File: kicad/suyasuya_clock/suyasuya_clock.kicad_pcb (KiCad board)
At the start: 2 copper layers, 66 x 78.7 mm, 33 parts, among them J1 Jack-DC, J2 Conn_Writer, J3 Conn_GPS, J4 USB_OUTPUT, Q1 2sk4017, SW1 RESET, U1 ATmega328-P, U2 BA50DD0T, U3 7803, Y1 Ceralock

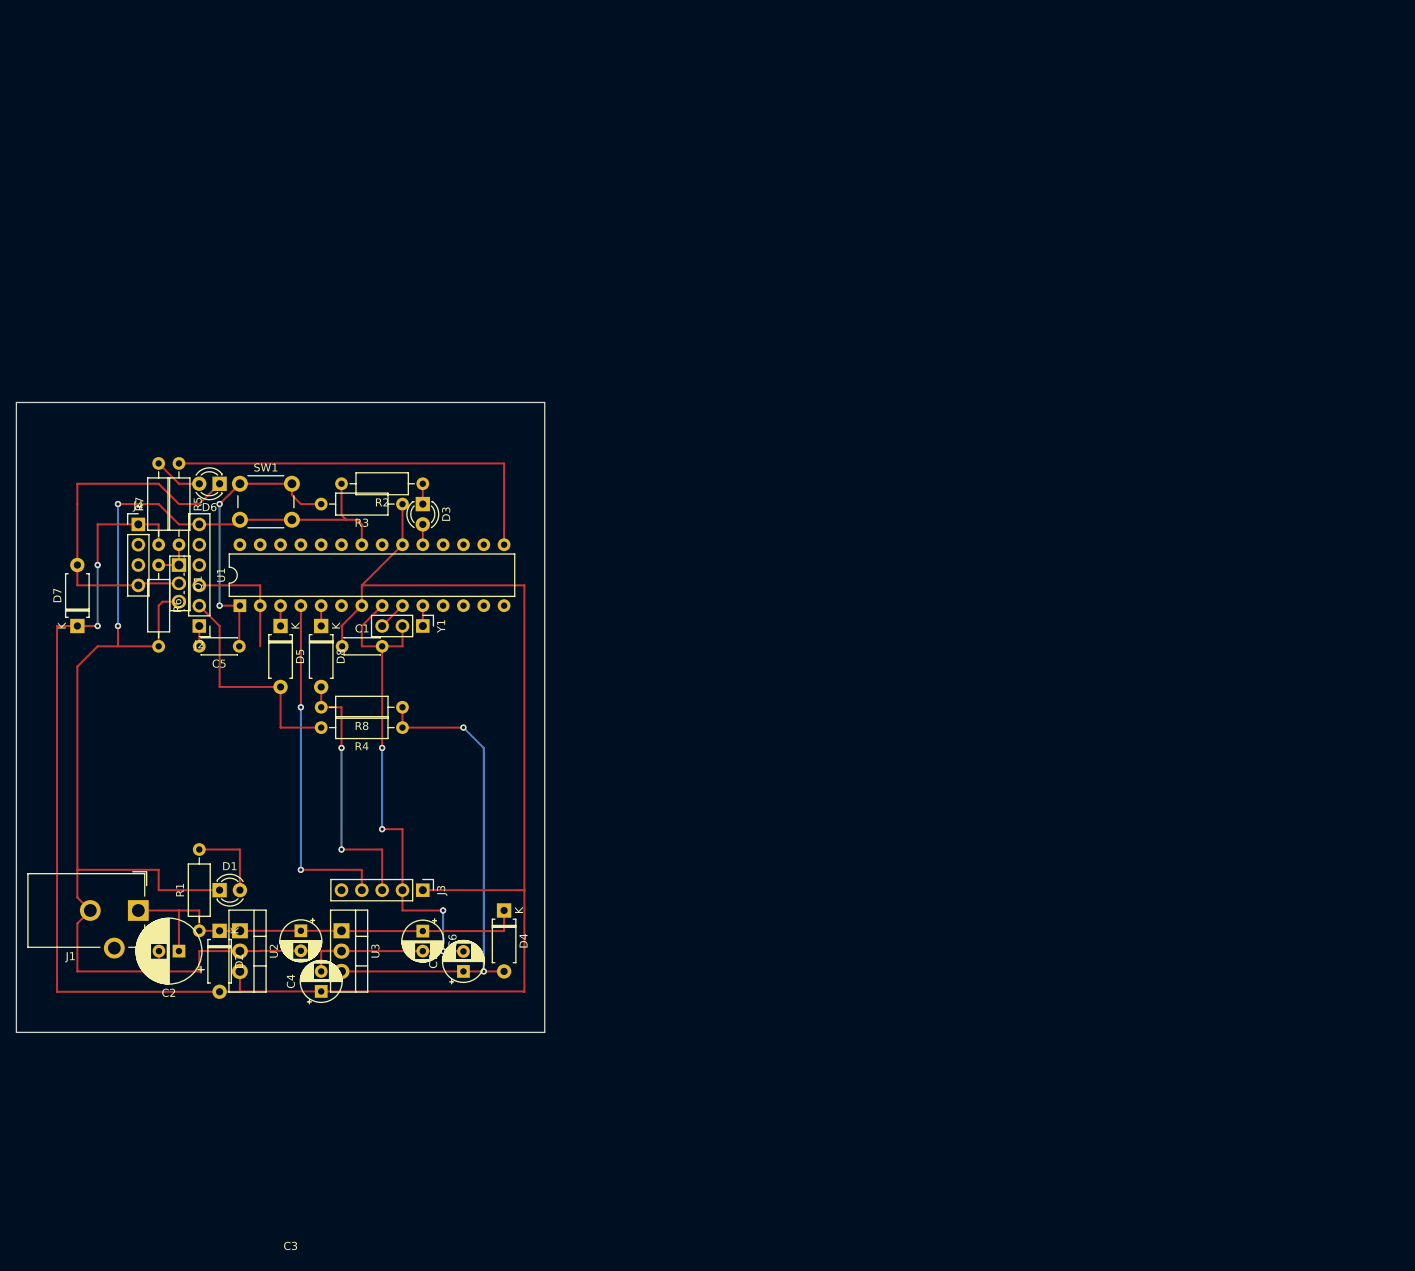
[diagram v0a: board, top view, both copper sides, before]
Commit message: アートワーク修正
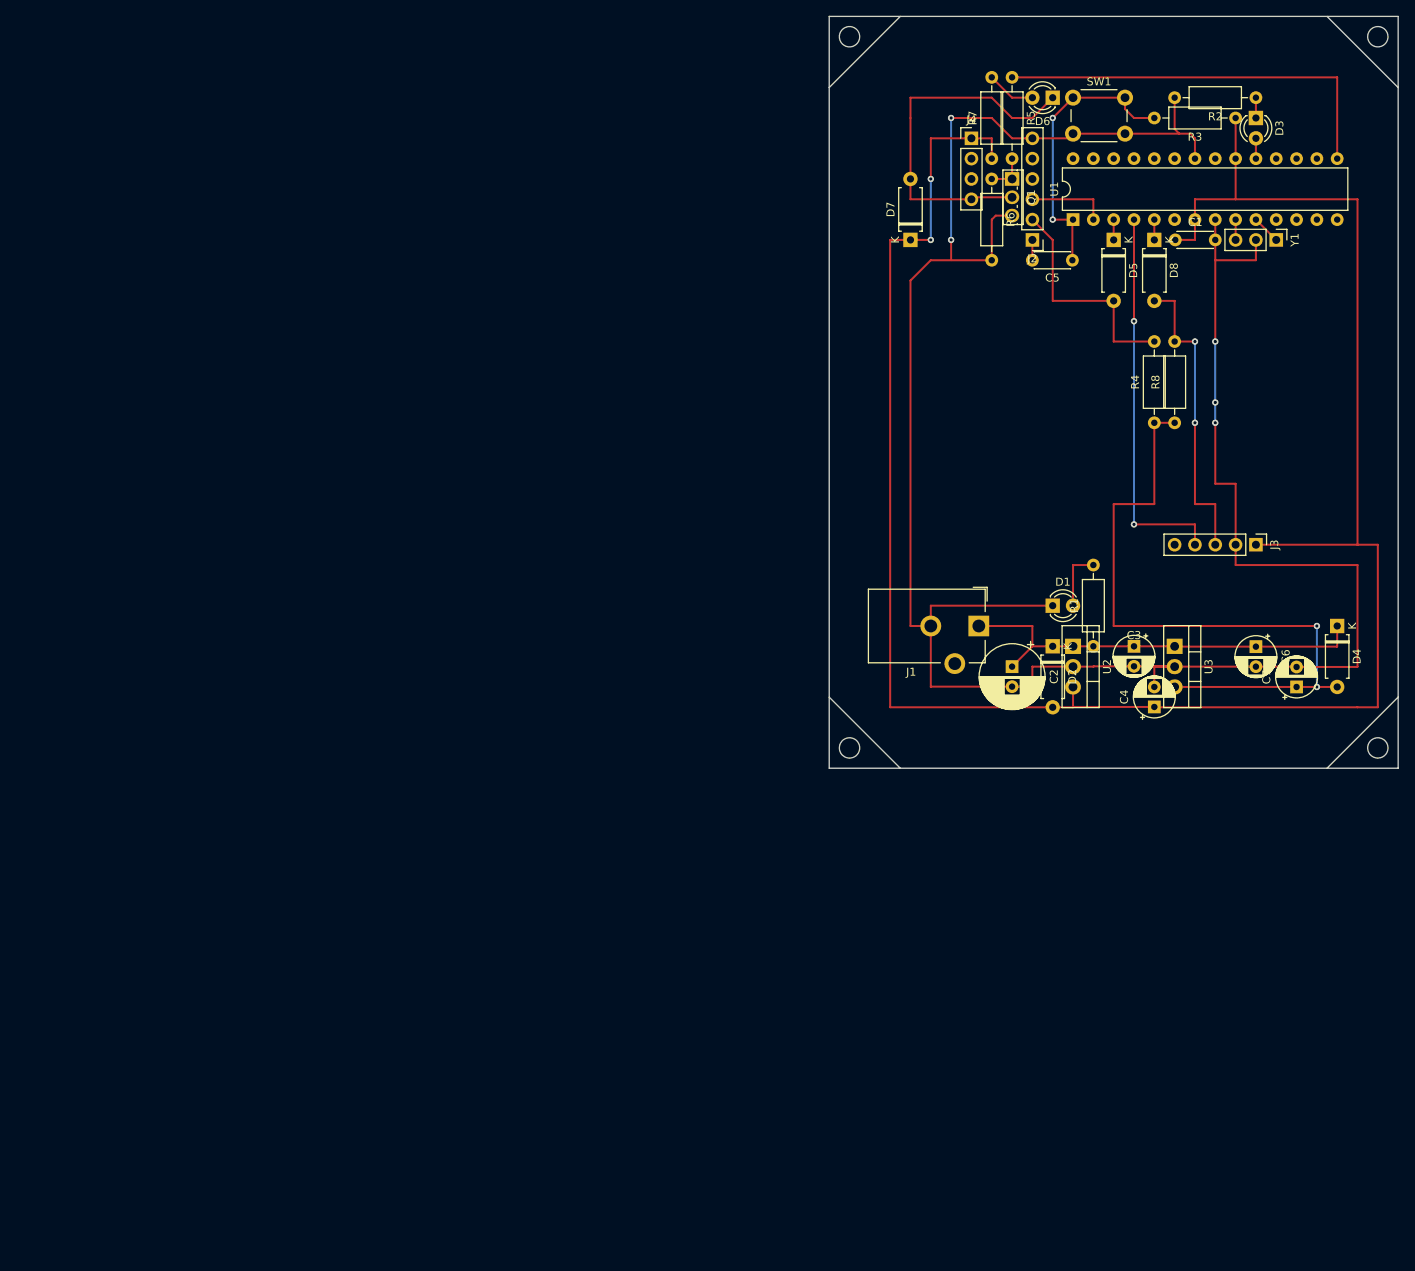
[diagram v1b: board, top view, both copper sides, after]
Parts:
- moved R1 117.3 mm to (208.3, 119.4)
- moved Y1 117.1 mm to (231.1, 68.6)
- moved C1 115.9 mm to (218.5, 68.6)
- moved R6 114.8 mm to (195.6, 61.0)
- moved R7 114.8 mm to (195.6, 58.4)
- moved SW1 114.8 mm to (205.7, 50.8)
- moved U1 114.8 mm to (205.7, 66.0)
- moved C5 114.8 mm to (205.7, 71.1)
- moved D3 114.8 mm to (228.6, 53.3)
- moved D8 114.8 mm to (215.9, 68.6)
- moved J2 114.8 mm to (200.7, 68.6)
- moved Q1 114.8 mm to (198.1, 61.0)
- moved R2 114.8 mm to (228.6, 50.8)
- moved R3 114.8 mm to (226.1, 53.3)
- moved R5 114.8 mm to (198.1, 48.3)
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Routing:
- net GND: track 253.8 -> 289.6 mm, vias 6 -> 5
- net +5V: track 239.4 -> 266.8 mm
- net +3V3: track 62.0 -> 86.4 mm
- net Net-(D8-Pad2): track 33.0 -> 38.1 mm
- net RX: track 15.2 -> 10.2 mm
- net GPS_RX: track 43.2 -> 48.3 mm
- net Net-(D1-Pad2): track 10.2 -> 7.62 mm
- net +12V: track 55.9 -> 53.5 mm
- net Net-(U1-Pad9): track 3.59 -> 2.54 mm
- net Net-(U1-Pad10): track 2.54 -> 3.59 mm
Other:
- board size 66 x 78.7 mm -> 71.1 x 94 mm
